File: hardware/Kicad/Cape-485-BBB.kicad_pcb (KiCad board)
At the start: 2 copper layers, 86.4 x 65.9 mm, 48 parts, among them J1 RJ25, J2 RJ25, P1 CONN_01X01, P10 CONN_02X05, Q1 BSR14, Q2 BSR14, Q3 BSR14, U1 MAX3107E, U3 IL3685, U4 DCR01XXXXU, U5 TS5A21366, U6 TS5A21366, X1 OSCILADOR

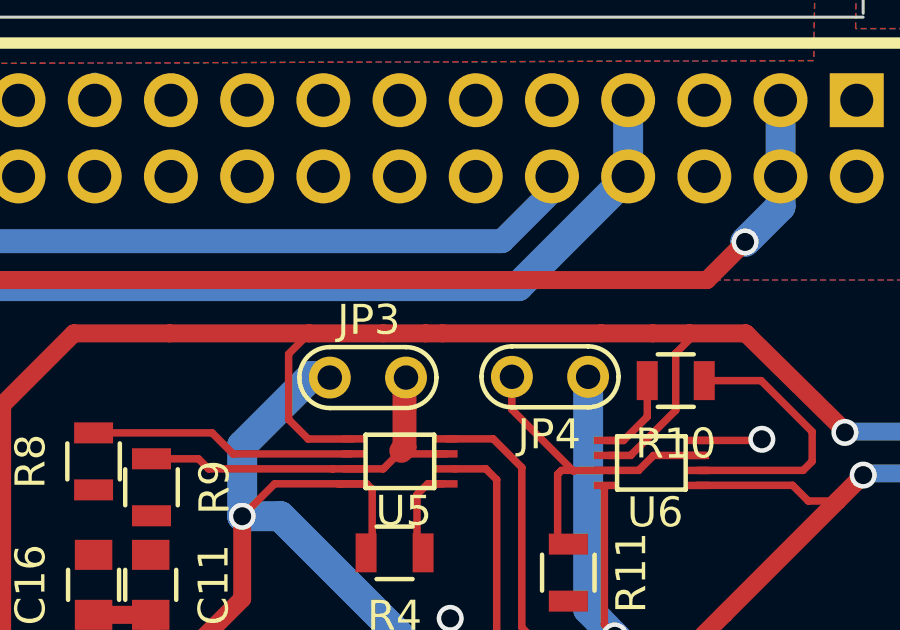
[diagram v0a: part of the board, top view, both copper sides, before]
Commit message: new hardware version
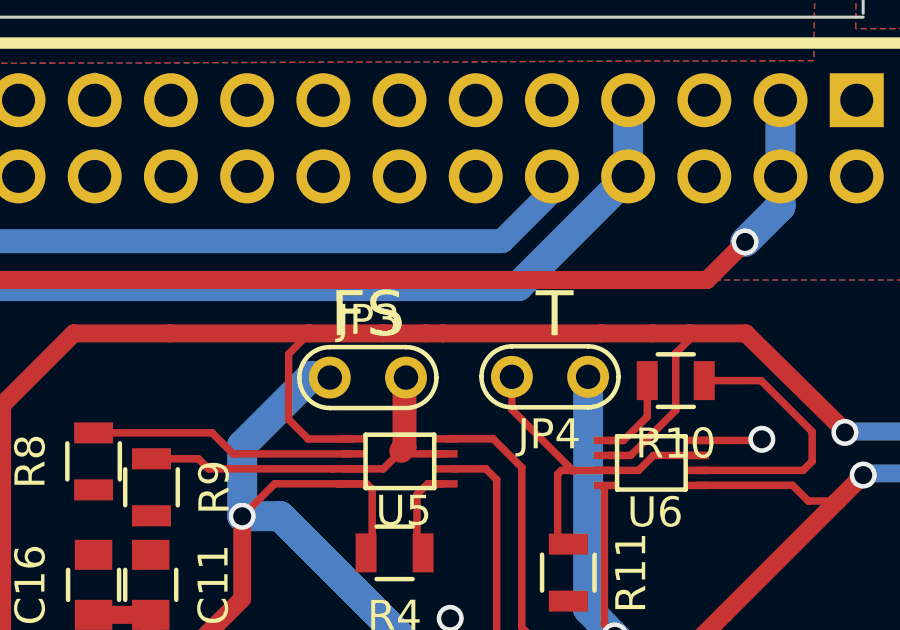
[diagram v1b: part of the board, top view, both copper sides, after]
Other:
- board text added: "FS"
- board text added: "T"
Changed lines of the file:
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@@
     (links 127)
     (no_connects 9)
-    (area 105.309999 67.386999 191.820001 133.384001)
+    (area 100.1014 65.8622 220.115566 136.042401)
     (thickness 1.6)
     (drawings 36)
@@
     (34 B.Paste user hide)
     (35 F.Paste user hide)
-    (36 B.SilkS user hide)
+    (36 B.SilkS user)
     (37 F.SilkS user)
     (38 B.Mask user hide)
@@
   )
   (setup
-    (last_trace_width 0.6)
+    (last_trace_width 0.4)
     (user_trace_width 0.25)
     (user_trace_width 0.6)
@@
     )
   )
+  (gr_text T (at 161.925 86.741) (layer F.SilkS)
+    (effects (font (size 1.5 1.5) (thickness 0.3)))
+  )
+  (gr_text FS (at 155.702 86.741) (layer F.SilkS)
+    (effects (font (size 1.5 1.5) (thickness 0.3)))
+  )
   (gr_line (start 116.967 76.835) (end 172.212 76.835) (angle 90) (layer Edge.Cuts) (width 0.1))
   (gr_line (start 191.77 67.437) (end 191.643 67.437) (angle 90) (layer Edge.Cuts) (width 0.1))
@@
     (effects (font (size 1 1) (thickness 0.25)))
   )
-  (dimension 14.176864 (width 0.3) (layer B.SilkS)
-    (gr_text "14,177 mm" (at 197.017062 92.768282 341.7273617) (layer B.SilkS)
-      (effects (font (size 1.5 1.5) (thickness 0.3)))
-    )
-    (feature1 (pts (xy 207.772 82.804) (xy 203.324785 96.272709)))
-    (feature2 (pts (xy 194.31 78.359) (xy 189.862785 91.827709)))
-    (crossbar (pts (xy 190.70934 89.263856) (xy 204.17134 93.708856)))
-    (arrow1a (pts (xy 204.17134 93.708856) (xy 202.917774 93.912504)))
-    (arrow1b (pts (xy 204.17134 93.708856) (xy 203.285506 92.798802)))
-    (arrow2a (pts (xy 190.70934 89.263856) (xy 191.595174 90.17391)))
-    (arrow2b (pts (xy 190.70934 89.263856) (xy 191.962906 89.060208)))
-  )
-  (dimension 6.14344 (width 0.3) (layer B.SilkS)
-    (gr_text "6,143 mm" (at 214.179851 90.177231 82.87498365) (layer B.SilkS)
-      (effects (font (size 1.5 1.5) (thickness 0.3)))
-    )
-    (feature1 (pts (xy 209.423 86.487) (xy 215.900426 87.296678)))
-    (feature2 (pts (xy 208.661 92.583) (xy 215.138426 93.392678)))
-    (crossbar (pts (xy 212.459276 93.057784) (xy 213.221276 86.961784)))
-    (arrow1a (pts (xy 213.221276 86.961784) (xy 213.663443 88.152325)))
-    (arrow1b (pts (xy 213.221276 86.961784) (xy 212.499658 88.006852)))
-    (arrow2a (pts (xy 212.459276 93.057784) (xy 213.180894 92.012716)))
-    (arrow2b (pts (xy 212.459276 93.057784) (xy 212.017109 91.867243)))
-  )
   (gr_text "Patrícia Nallin\n\nCONTROLE 2016" (at 108.9152 105.2068 270) (layer B.Cu)
